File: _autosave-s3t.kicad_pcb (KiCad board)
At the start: 2 copper layers, 134 x 80 mm, 65 parts, among them J1 DEBUG_UART0, J2 Conn_01x02, J3 USB_OTG, J4 HOLE, J5 HOLE, J6 HOLE, J7 HOLE, SW1 SW_DIP_x01, SW2 SW_DIP_x01, SW3 SW_DIP_x01, SW4 SW_DIP_x01, SW5 SW_DIP_x01, SW6 SW_DIP_x01, U1 AMS1117-3.3, U2 TF_CARD, U3 s3core, U4 SX1308, U5 PT4103, U6 THERMAL, U7 LCD_A050FW01

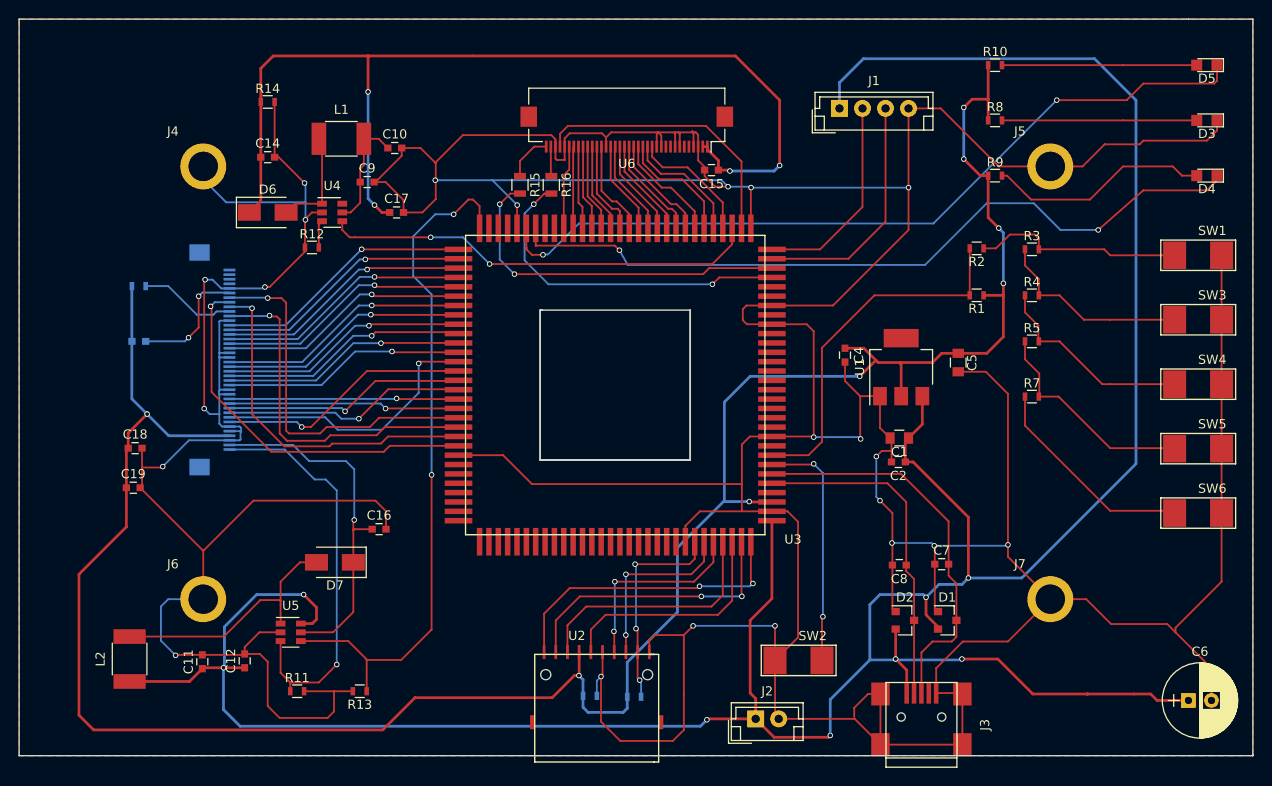
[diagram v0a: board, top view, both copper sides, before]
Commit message: finish all pcb and send to factory
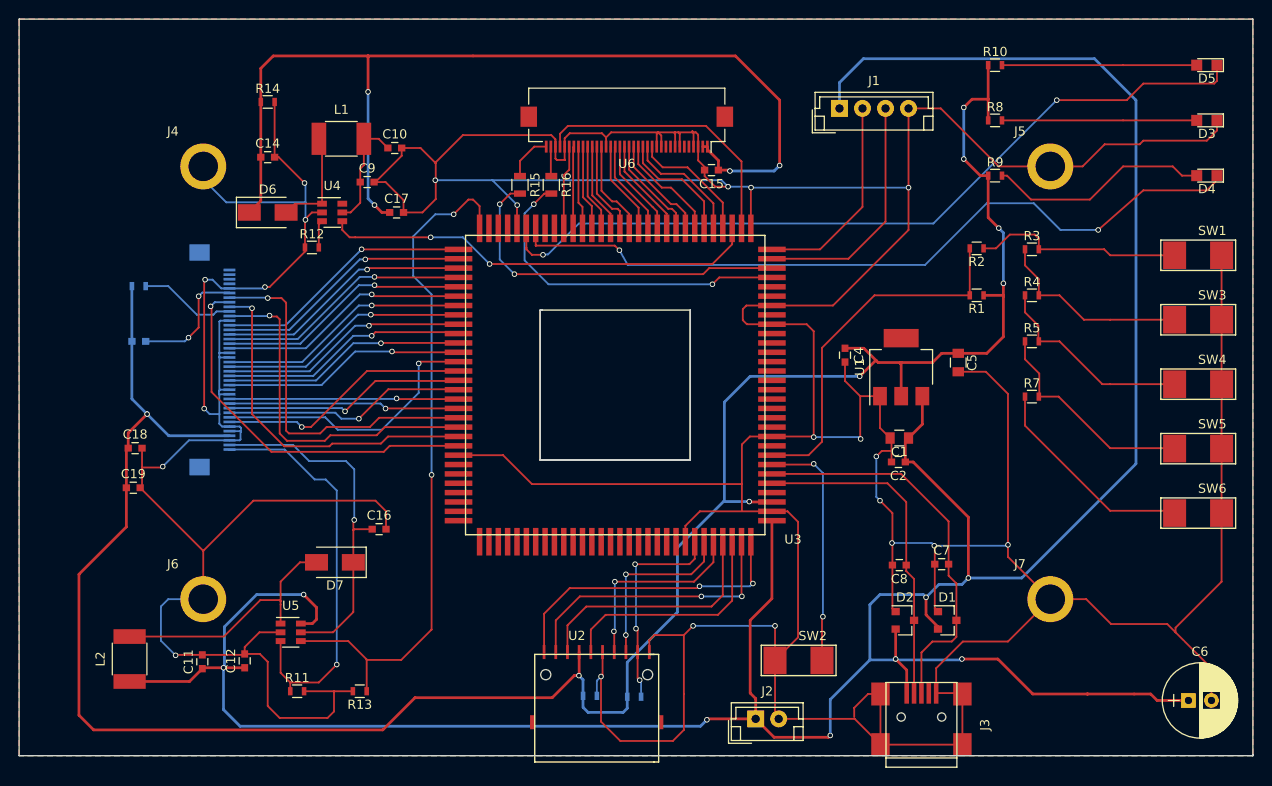
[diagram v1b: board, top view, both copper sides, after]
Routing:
- added copper zone on B.Cu, net GND
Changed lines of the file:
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@@
     (links 203)
     (no_connects 0)
-    (area 50.150002 34.8 202.075001 152.7)
+    (area 67.924999 57.924999 202.075001 138.075001)
     (thickness 1.6)
     (drawings 18)
@@
     (visible_elements 7FFFFFFF)
     (pcbplotparams
-      (layerselection 0x00030_80000001)
+      (layerselection 0x03fff_80000001)
       (usegerberextensions false)
       (excludeedgelayer true)
@@
       (outputformat 1)
       (mirror false)
-      (drillshape 1)
+      (drillshape 0)
       (scaleselection 1)
-      (outputdirectory ""))
+      (outputdirectory s3t-gerber))
   )
   (net 0 "")
@@
     (connect_pads (clearance 0.508))
     (min_thickness 0.254)
+    (fill yes (arc_segments 16) (thermal_gap 0.508) (thermal_bridge_width 0.508))
+    (polygon
+      (pts
+        (xy 202 138) (xy 68 138) (xy 68 58) (xy 202 58)
+      )
+    )
+  )
+  (zone (net 0) (net_name "") (layer B.Cu) (hatch edge 0.508)
+    (connect_pads (clearance 0.508))
+    (min_thickness 0.254)
+    (keepout (tracks not_allowed) (vias allowed) (copperpour not_allowed))
+    (fill (arc_segments 16) (thermal_gap 0.508) (thermal_bridge_width 0.508))
+    (polygon
+      (pts
+        (xy 140.9 105.9) (xy 124.6 105.9) (xy 124.6 89.6) (xy 140.9 89.6)
+      )
+    )
+  )
+  (zone (net 2) (net_name GND) (layer B.Cu) (hatch edge 0.508)
+    (connect_pads (clearance 0.508))
+    (min_thickness 0.254)
